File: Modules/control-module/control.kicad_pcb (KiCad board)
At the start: 4 copper layers, 150.6 x 117.1 mm, 46 parts, among them J12 Conn_01x04, J2 Screw_Terminal_01x04, J3 Conn_01x25, J4 Screw_Terminal_01x04, J5 Conn_01x03, J50 Screw_Terminal_01x02, J8 Conn_01x08, SW6 SW_Push, U1 74LS161, U2 74LS173, U3 74LS245, U4 74LS173, U5 74LS173, U6 74LS138, U7 74LS04, U8 74LS138

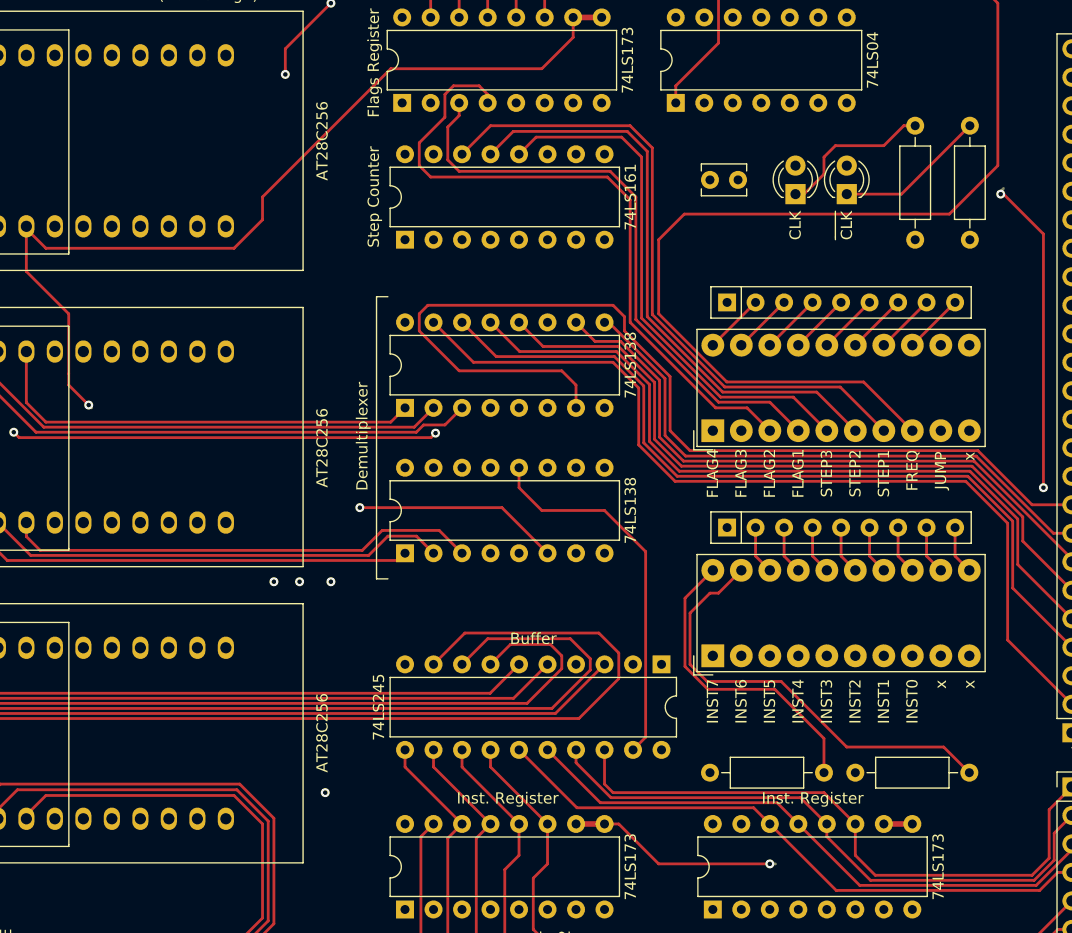
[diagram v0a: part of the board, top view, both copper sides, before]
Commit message: [Micocode] Updating Control - WIP
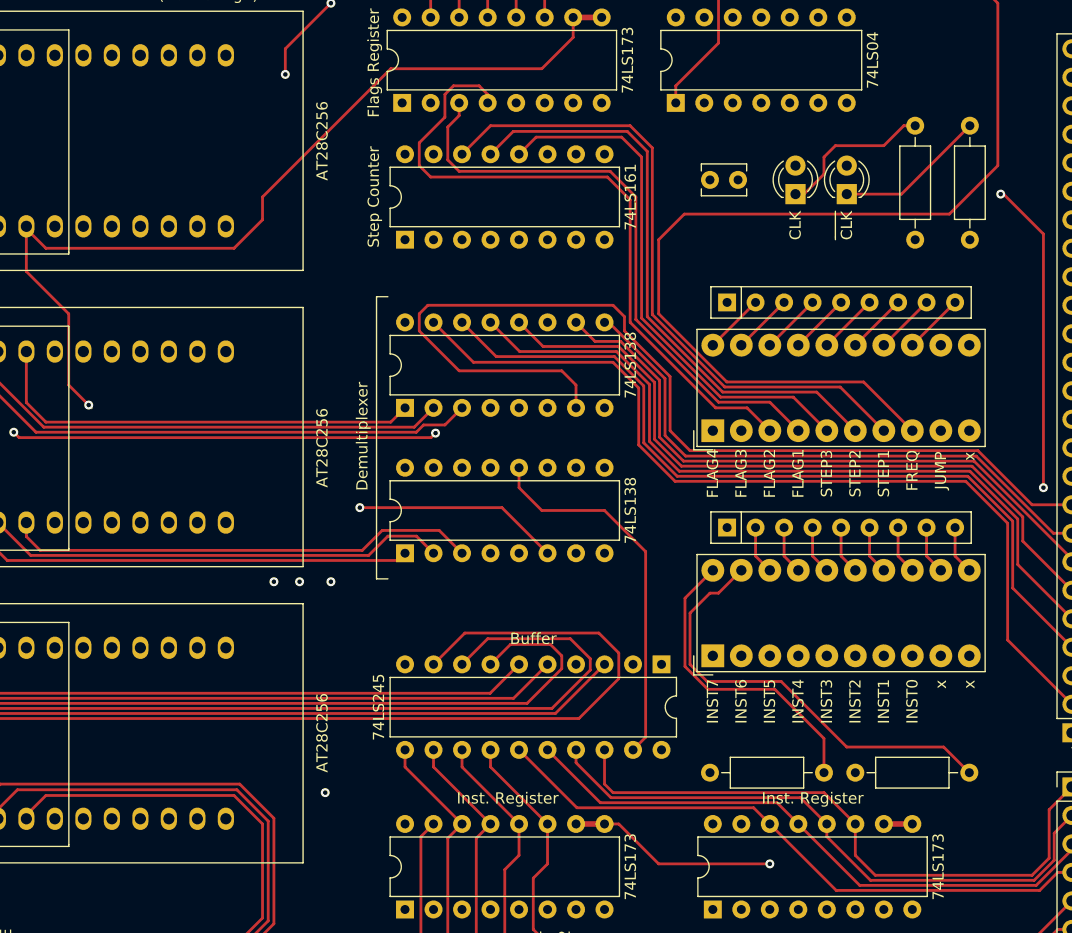
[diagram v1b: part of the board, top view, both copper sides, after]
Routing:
- net CLOCK: track 179.1 -> 178.0 mm
- net INSTRUCTION_REG_IN: track 181.9 -> 181.3 mm
- net FLAG4: track 203.0 -> 202.5 mm
